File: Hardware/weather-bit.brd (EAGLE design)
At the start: 68.6 x 63.5 mm, 41 parts, among them J1 EDGE-80PTH-RA, J2 RJ11, J3 RJ11, U1 BME280

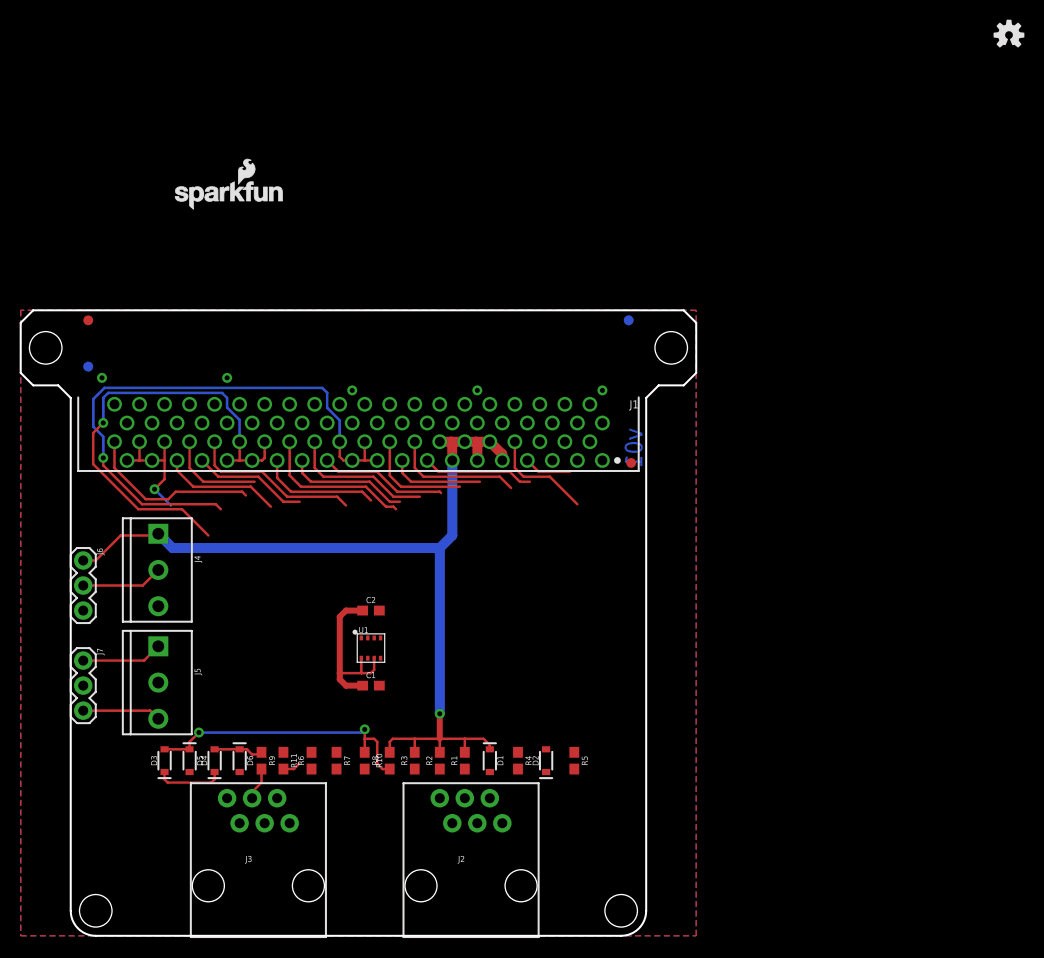
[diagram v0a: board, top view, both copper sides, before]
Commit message: Updated Baord Layout, prepping for today's meeting
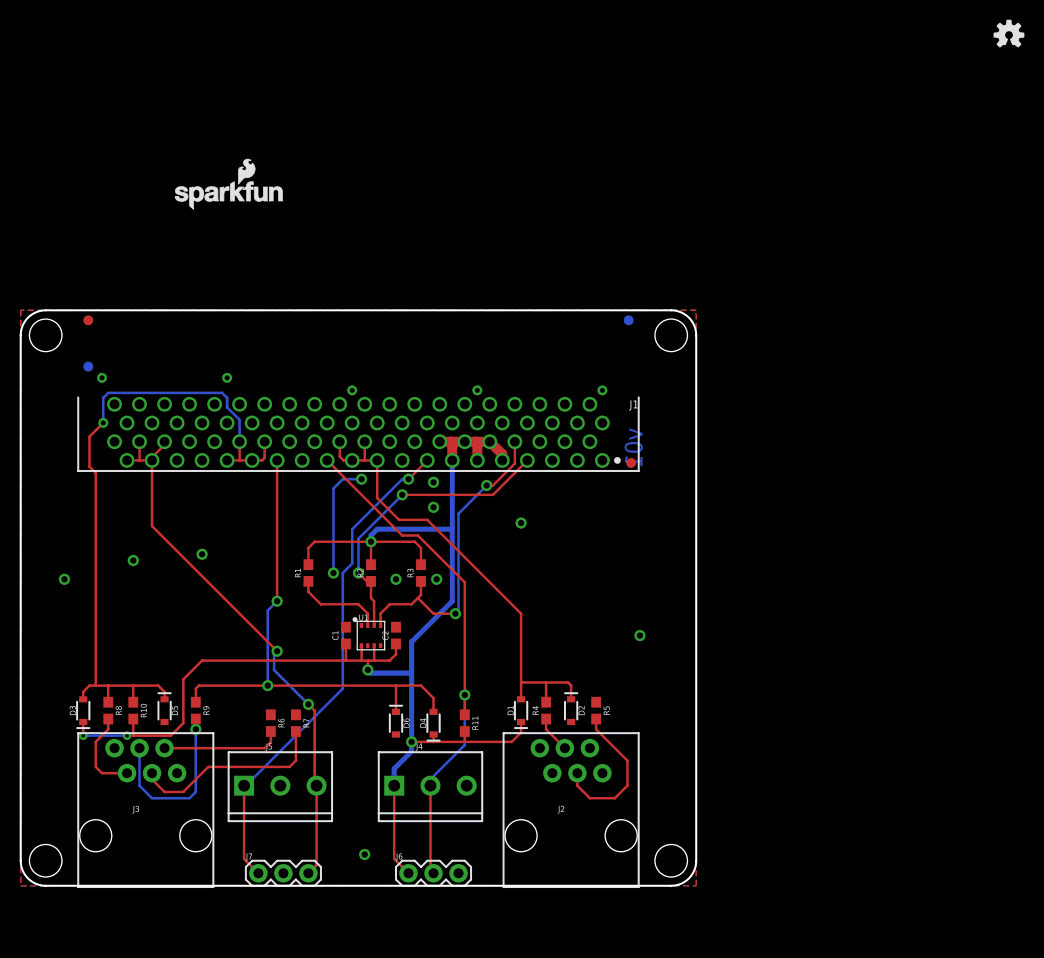
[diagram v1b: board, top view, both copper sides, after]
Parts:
- moved J6 45.8 mm to (39.4, 6.35), turned to 0 degrees
- moved J4 35.0 mm to (38.1, 15.2), turned to 0 degrees
- moved J7 28.0 mm to (24.1, 6.35), turned to 0 degrees
- moved R10 26.5 mm to (11.4, 22.9), turned to 270 degrees
- moved R8 26.5 mm to (8.89, 22.9)
- moved R1 24.8 mm to (29.2, 36.8)
- moved D4 22.5 mm to (41.9, 21.6)
- moved R2 20.3 mm to (35.6, 36.8)
- moved R3 19.1 mm to (40.6, 36.8)
- moved R11 18.8 mm to (45.1, 21.6)
- moved J5 16.6 mm to (22.9, 15.2), turned to 0 degrees
- moved D6 16.3 mm to (38.1, 21.6)
- moved J3 12.5 mm to (12.7, 10.2)
- moved J2 11.4 mm to (55.9, 10.2)
- moved D3 9.69 mm to (6.35, 22.9)
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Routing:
- net WSPEED: track 17.3 -> 53.5 mm, vias 0 -> 2
- net SOIL_DAT: track 21.2 -> 56.5 mm, vias 1 -> 2
- net SOIL_PWR: track 19.5 -> 50.7 mm, vias 0 -> 1
- net TEMP_DAT: track 21.2 -> 52.2 mm, vias 0 -> 1
- net 3.3V: track 120.8 -> 149.9 mm, vias 1 -> 5
- net SDA: track 4.79 -> 30.3 mm, vias 0 -> 2
- net SCL: track 10.5 -> 32.3 mm, vias 0 -> 2
- net N$14: track 0.00 -> 20.0 mm
- net 3: track 17.8 -> 0.00 mm
- net 7: track 17.4 -> 0.00 mm
- net 9: track 15.6 -> 0.00 mm
- net N$7: track 0.00 -> 15.5 mm
- net 11: track 14.5 -> 0.00 mm
- net N$11: track 3.35 -> 17.7 mm, vias 0 -> 1
- net 15: track 13.3 -> 0.00 mm
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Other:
- board size 68.6 x 63.5 mm -> 68.6 x 58.4 mm
